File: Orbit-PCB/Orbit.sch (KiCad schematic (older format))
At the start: 294 parts, among them J1 PJ-3200B-4A, J10 Breakaway_Tabs, J11 PJ-3200B-4A, J12 AVR-ISP-6, J13 Breakaway_Tabs, J14 Breakaway_Tabs, J17 Breakaway_Tabs, J18 Breakaway_Tabs, J19 Breakaway_Tabs, J2 AVR-ISP-6, J20 Breakaway_Tabs, J3 Breakaway_Tabs, J5 Breakaway_Tabs, J6 Breakaway_Tabs, J7 Breakaway_Tabs, J9 Breakaway_Tabs, Q1 2N7002, Q2 2N7002, SW1 SW_Push, SW2 SW_Push, U1 ATmega32U4-MU, U2 PRTR5V0U2X, U3 ATmega32U4-MU, U4 PRTR5V0U2X, Y1 16MHz, Y2 16MHz

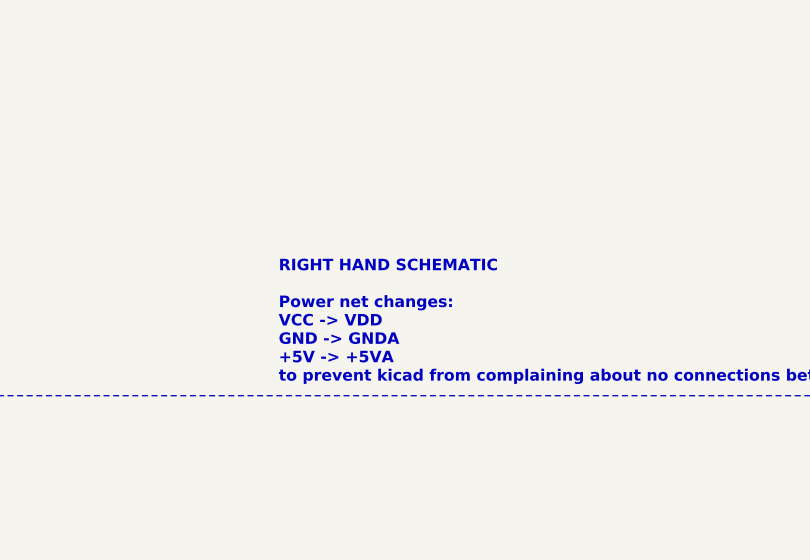
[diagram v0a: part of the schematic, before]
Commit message: Add a comment
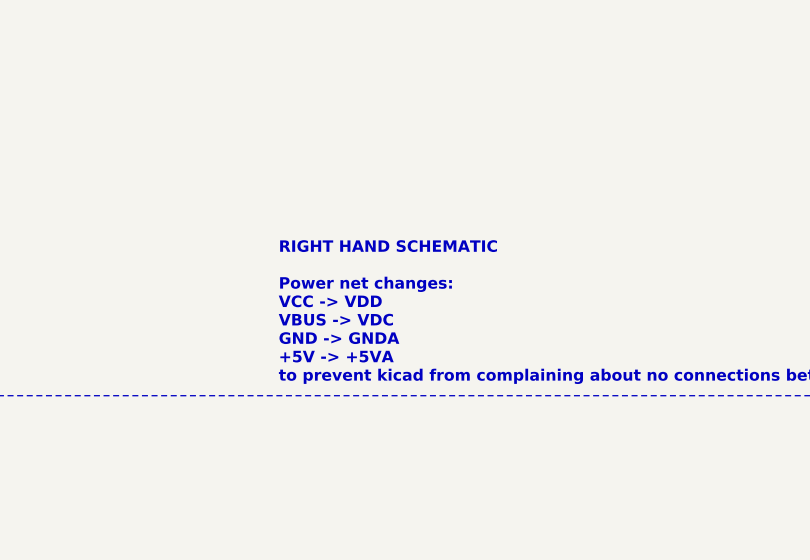
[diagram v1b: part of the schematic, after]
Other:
- note added: "RIGHT HAND SCHEMATIC\n\nPower net changes:\nVCC -> VDD\nVBUS -> VDC\nGND -> GNDA\n+5V -> +5VA\nto prevent kicad from complaining about no connections between halves"
- note removed: "RIGHT HAND SCHEMATIC\n\nPower net changes:\nVCC -> VDD\nGND -> GNDA\n+5V -> +5VA\nto prevent kicad from complaining about no connections between halves"
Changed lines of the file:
@@
 LEFT HAND SCHEMATIC
 Text Notes 11100 15225 0    50   ~ 10
-RIGHT HAND SCHEMATIC\n\nPower net changes:\nVCC -> VDD\nGND -> GNDA\n+5V -> +5VA\nto prevent kicad from complaining about no connections between halves
+RIGHT HAND SCHEMATIC\n\nPower net changes:\nVCC -> VDD\nVBUS -> VDC\nGND -> GNDA\n+5V -> +5VA\nto prevent kicad from complaining about no connections between halves
 $Comp
 L power:VDD #PWR0123

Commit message: Generate 2.1 production data
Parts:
- Y1, Y2: footprint Crystals:Crystal_SMD_2520-4pin_2.5x2.0mm -> Crystals:Crystal_SMD_3225-4pin_3.2x2.5mm
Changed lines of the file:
@@
 F 0 "Y1" V 2479 1816 50  0000 L CNN
 F 1 "16MHz" V 2570 1816 50  0000 L CNN
-F 2 "Crystals:Crystal_SMD_2520-4pin_2.5x2.0mm" H 2525 1650 50  0001 C CNN
+F 2 "Crystals:Crystal_SMD_3225-4pin_3.2x2.5mm" H 2525 1650 50  0001 C CNN
 F 3 "~" H 2525 1650 50  0001 C CNN
 	1    2525 1650
@@
 F 0 "Y2" V 2479 9391 50  0000 L CNN
 F 1 "16MHz" V 2570 9391 50  0000 L CNN
-F 2 "Crystals:Crystal_SMD_2520-4pin_2.5x2.0mm" H 2525 9225 50  0001 C CNN
+F 2 "Crystals:Crystal_SMD_3225-4pin_3.2x2.5mm" H 2525 9225 50  0001 C CNN
 F 3 "~" H 2525 9225 50  0001 C CNN
 	1    2525 9225
